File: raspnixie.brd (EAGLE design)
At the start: 87.6 x 58.5 mm, 30 parts, among them IC1 74141N, IC2 74141N, IC3 74141N, IC4 74141N, T1 IRF644B, T2 13001, U1 ZM1000, U2 ZM1000, U3 ZM1000, U4 ZM1000, U5 MAX1771CPA+, X1 RASPI_BOARD_B+#_E3P

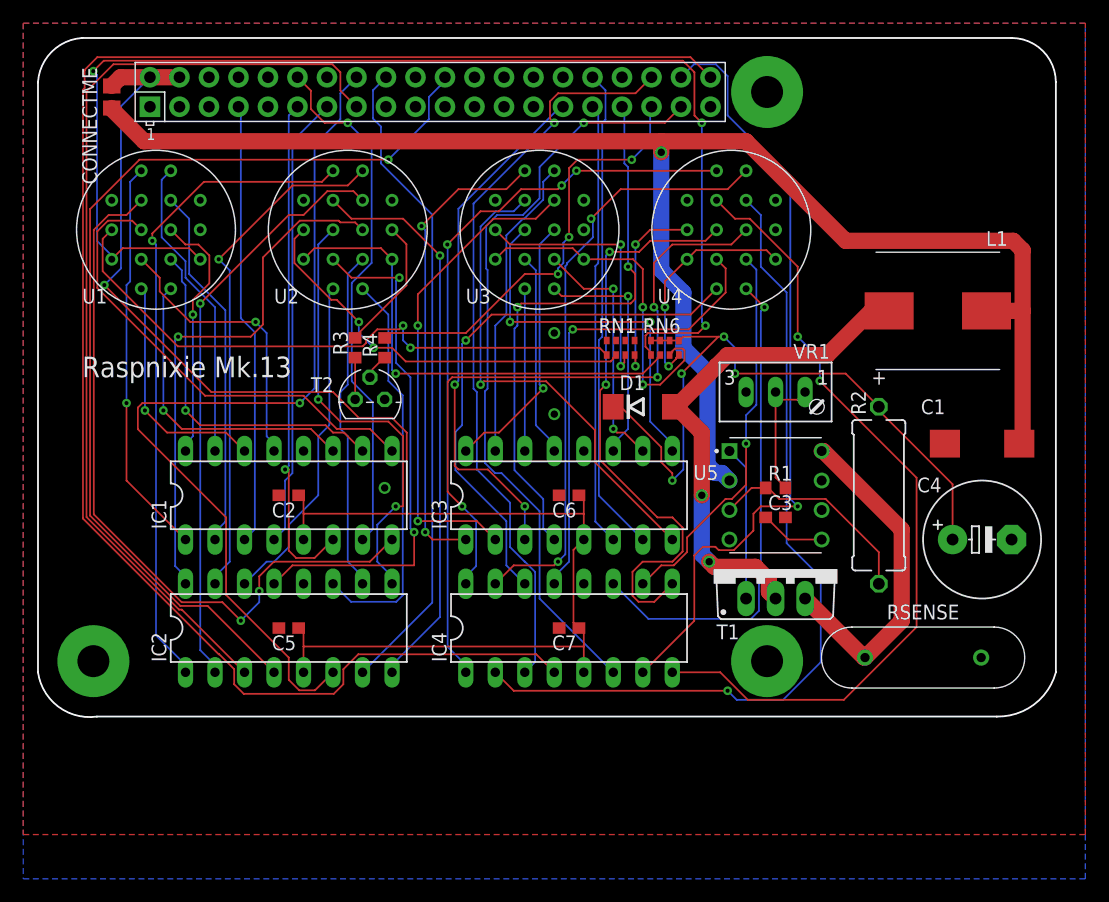
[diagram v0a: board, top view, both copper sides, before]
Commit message: mark. 14
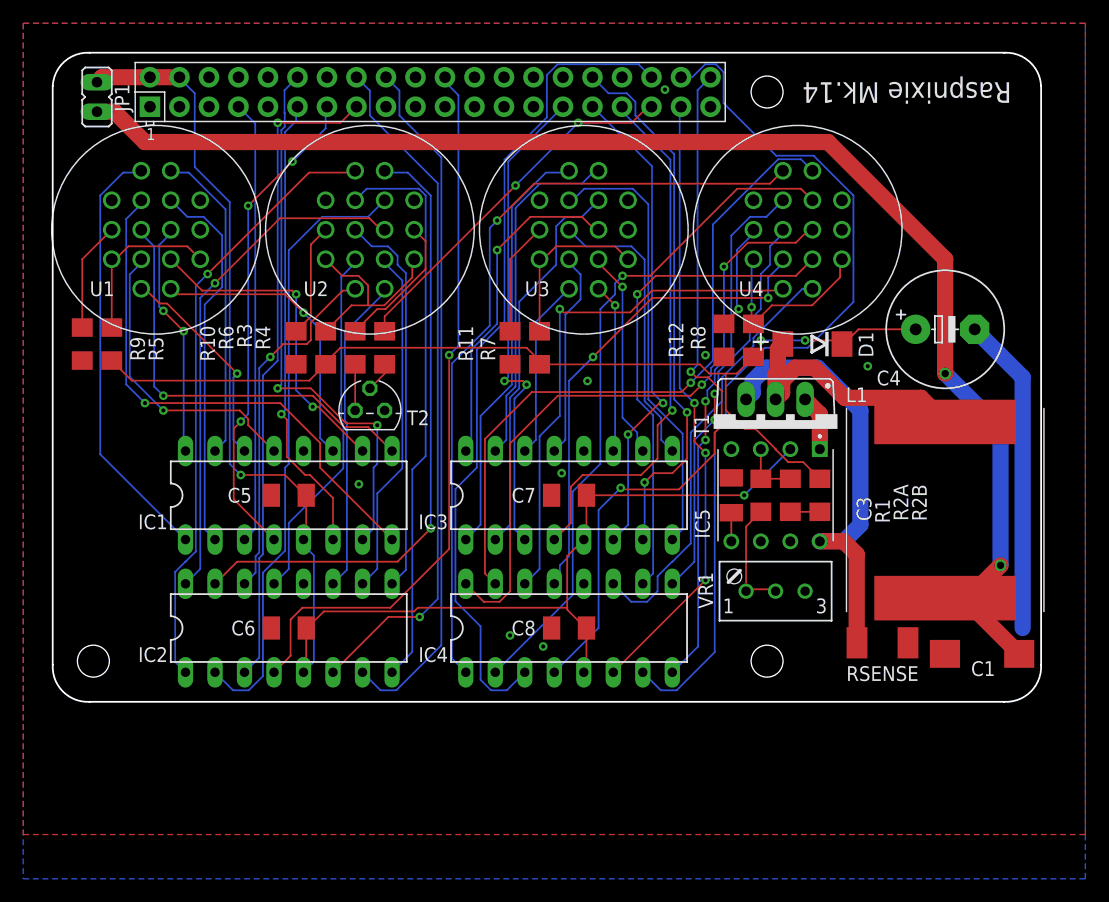
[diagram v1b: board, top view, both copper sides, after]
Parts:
- removed C2: 10n, rcl:C0603
- removed CONNECTME: 0, rcl:R0805
- removed R2: 1M5, rcl:P0613/15
- removed RN1: 10M, resistor-dil:0603-ARC
- removed RN6: 18k, resistor-dil:0603-ARV
- added C8: 10n, rcl:C1206K
- added JP1: (no value), jumper:JP1
- added R10, R11, R12, R9: 10M, rcl:R1206
- added R2A, R2B: 750k, rcl:R1206
- added R5, R6, R7, R8: 15k, rcl:R1206
- C3, C5, C6, C7: device rcl:C0603 -> rcl:C1206K
- L1: value 101 -> 221; device raspnixie:INDM106101X500N -> raspnixie:RESM175170X700N
- R1, R3, R4: device rcl:R0603 -> rcl:R1206
- RSENSE: device raspnixie:XTALRR1000W60L1750T525H1800B -> rcl:R2010
- VR1: device pot:S64W -> pot-hex:S64W-ROUND
- X1: value RASPI_BOARD_B+#_E3P -> RASPI_BOARD_B+#_E3; device raspberrypi_bastelstube_v13:RASPI_BOARD_B+_EDGES_3DRILL_PAD -> raspberrypi_bastelstube_v13:RASPI_BOARD_B+_EDGES_3DRILL
- moved C6 26.7 mm to (21.6, 7.62)
- moved C4 18.4 mm to (78.1, 33.3)
- moved C1 18.1 mm to (81.3, 5.40)
- moved L1 17.2 mm to (78.1, 17.8), turned to 90 degrees
- moved D1 15.6 mm to (66.7, 32.1), turned to 180 degrees
- moved VR1 14.6 mm to (63.5, 12.1), turned to 180 degrees
- moved T1 12.1 mm to (63.5, 24.8), turned to 180 degrees
- moved C5 11.4 mm to (21.6, 19.1)
- moved C7 11.4 mm to (45.7, 19.1)
- moved U4 5.72 mm to (65.4, 41.9)
- moved C3 4.26 mm to (59.7, 19.1), turned to 90 degrees
- moved U3 3.81 mm to (47.0, 41.9)
- moved RSENSE 3.72 mm to (72.7, 6.35)
- moved U2 1.90 mm to (28.6, 41.9)
- moved R1 1.42 mm to (62.2, 19.1), turned to 270 degrees
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- renumbered U5 to IC5
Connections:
- new net N$75: R2A.2, R2B.1
- net GND: now also C8.2, R10.2, R11.2, R12.2, R9.2; no longer C2.2, RN1.5, RN1.6, RN1.7, RN1.8
- net N$1: now also R9.1; no longer RN1.1
- net N$2: now also R10.1; no longer RN1.2
- net N$3: now also R11.1; no longer RN1.3
- net N$4: now also R12.1; no longer RN1.4
- net N$65: now also R5.1; no longer RN6.1
- net N$66: now also R6.1; no longer RN6.2
- net N$70: now also R2A.1; no longer R2.2
- net N$71: now also R7.1; no longer RN6.3
- net N$72: now also R8.1; no longer RN6.4
- net V+: now also JP1.1; no longer CONNECTME.2, IC5.2
- net VCC: now also C8.1, IC5.2, JP1.2; no longer C2.1, CONNECTME.1
- net VH: now also R2B.2, R5.2, R6.2, R7.2, R8.2; no longer R2.1, RN6.5, RN6.6, RN6.7, RN6.8
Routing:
- net N$65: track 107.4 -> 14.4 mm, vias 3 -> 0
- net N$60: track 144.3 -> 62.7 mm, vias 0 -> 2
- net N$1: track 52.6 -> 9.47 mm, vias 2 -> 0
- net VH: track 60.6 -> 89.1 mm, vias 4 -> 2
- net GND: track 0.08 -> 27.4 mm, vias 3 -> 8
- net N$64: track 82.4 -> 55.8 mm, vias 0 -> 1
- net N$2: track 35.2 -> 9.79 mm, vias 2 -> 0
- net N$66: track 41.9 -> 17.3 mm, vias 1 -> 0
- net N$38: track 69.2 -> 45.4 mm
- net N$52: track 84.4 -> 62.7 mm
- net N$62: track 44.2 -> 23.3 mm, vias 2 -> 0
- net N$50: track 77.8 -> 59.4 mm
- net N$8: track 63.3 -> 46.1 mm, vias 2 -> 1
- net N$39: track 51.2 -> 34.4 mm
- net N$71: track 30.7 -> 14.7 mm, vias 2 -> 0
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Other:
- board size 87.6 x 58.5 mm -> 85.1 x 55.9 mm
- board text added: "Raspnixie Mk.14"
- board text removed: "Raspnixie Mk.13"

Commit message: steal from other libraries
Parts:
- IC1, IC2, IC3, IC4: device 74xx-eu:DIL16 -> raspnixie:DIL16
- IC5: device MAX1771CPA:DIP794W47P254L991H457Q8 -> raspnixie:DIP794W47P254L991H457Q8
- T1: device Transistor:TO220BV -> transistor-power:TO220BV
- T2: value 13001 -> A42; device Transistor:TO92 -> transistor:TO92
- VR1: device pot-hex:S64W-ROUND -> raspnixie:S64W-ROUND
- X1: device raspberrypi_bastelstube_v13:RASPI_BOARD_B+_EDGES_3DRILL -> raspnixie:RASPI_BOARD_B+_EDGES_3DRILL
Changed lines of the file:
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@@
 <drawing>
 <settings>
-<setting alwaysvectorfont="yes"/>
+<setting alwaysvectorfont="no"/>
 <setting verticaltext="up"/>
 </settings>
@@
 </autorouter>
 <elements>
-<element name="X1" library="raspberrypi_bastelstube_v13" package="RASPI_BOARD_B+_EDGES_3DRILL" value="RASPI_BOARD_B+#_E3" x="1.27" y="1.27" smashed="yes">
+<element name="X1" library="raspnixie" package="RASPI_BOARD_B+_EDGES_3DRILL" value="RASPI_BOARD_B+#_E3" x="1.27" y="1.27" smashed="yes">
 <attribute name="SPICEPREFIX" value="X" x="1.27" y="1.27" size="1.778" layer="27" display="off"/>
 </element>
-<element name="IC1" library="74xx-eu" library_urn="urn:adsk.eagle:library:85" package="DIL16" package3d_urn="urn:adsk.eagle:package:922/2" value="74141N" x="21.59" y="19.05" smashed="yes">
+<element name="IC1" library="raspnixie" package="DIL16" package3d_urn="urn:adsk.eagle:package:922/2" value="74141N" x="21.59" y="19.05" smashed="yes">
 <attribute name="NAME" x="11.176" y="17.399" size="1.27" layer="25" ratio="10" rot="R180"/>
 <attribute name="POPULARITY" value="0" x="21.59" y="34.29" size="1.778" layer="27" display="off"/>
@@
 <attribute name="NAME" x="4.445" y="36.195" size="1.27" layer="21"/>
 </element>
-<element name="IC2" library="74xx-eu" library_urn="urn:adsk.eagle:library:85" package="DIL16" package3d_urn="urn:adsk.eagle:package:922/2" value="74141N" x="21.59" y="7.62" smashed="yes">
+<element name="IC2" library="raspnixie" package="DIL16" package3d_urn="urn:adsk.eagle:package:922/2" value="74141N" x="21.59" y="7.62" smashed="yes">
 <attribute name="NAME" x="11.176" y="5.969" size="1.27" layer="25" ratio="10" rot="R180"/>
 <attribute name="POPULARITY" value="0" x="21.59" y="21.59" size="1.778" layer="27" display="off"/>
@@
 <attribute name="NAME" x="22.86" y="36.195" size="1.27" layer="21"/>
 </element>
-<element name="IC3" library="74xx-eu" library_urn="urn:adsk.eagle:library:85" package="DIL16" package3d_urn="urn:adsk.eagle:package:922/2" value="74141N" x="45.72" y="19.05" smashed="yes">
+<element name="IC3" library="raspnixie" package="DIL16" package3d_urn="urn:adsk.eagle:package:922/2" value="74141N" x="45.72" y="19.05" smashed="yes">
 <attribute name="NAME" x="35.306" y="17.399" size="1.27" layer="25" ratio="10" rot="R180"/>
 <attribute name="POPULARITY" value="0" x="45.72" y="33.02" size="1.778" layer="27" display="off"/>
@@
 <attribute name="NAME" x="41.91" y="36.195" size="1.27" layer="21"/>
 </element>
-<element name="IC4" library="74xx-eu" library_urn="urn:adsk.eagle:library:85" package="DIL16" package3d_urn="urn:adsk.eagle:package:922/2" value="74141N" x="45.72" y="7.62" smashed="yes">
+<element name="IC4" library="raspnixie" package="DIL16" package3d_urn="urn:adsk.eagle:package:922/2" value="74141N" x="45.72" y="7.62" smashed="yes">
 <attribute name="NAME" x="35.306" y="5.969" size="1.27" layer="25" ratio="10" rot="R180"/>
 <attribute name="POPULARITY" value="0" x="45.72" y="21.59" size="1.778" layer="27" display="off"/>
@@
 <attribute name="NAME" x="60.325" y="36.195" size="1.27" layer="21"/>
 </element>
-<element name="IC5" library="MAX1771CPA" package="DIP794W47P254L991H457Q8" value="MAX1771CPA+" x="63.5" y="19.05" smashed="yes" rot="R270">
+<element name="IC5" library="raspnixie" package="DIP794W47P254L991H457Q8" value="MAX1771CPA+" x="63.5" y="19.05" smashed="yes" rot="R270">
 <attribute name="AVAILABILITY" value="Unavailable" x="63.5" y="19.05" size="1.778" layer="27" rot="R270" display="off"/>
 <attribute name="DESCRIPTION" value=" Boost, Buck-Boost Regulator Positive Output Step-Up, Step-Up/Step-Down DC-DC Controller IC 8-PDIP " x="63.5" y="19.05" size="1.778" layer="27" rot="R270" display="off"/>
@@
 <attribute name="VALUE" x="83.82" y="9.2075" size="1.27" layer="27" rot="R180"/>
 </element>
-<element name="T1" library="Transistor" library_urn="urn:adsk.eagle:library:16378713" package="TO220BV" package3d_urn="urn:adsk.eagle:package:29484/3" value="IRF644B" x="63.5" y="24.765" smashed="yes" rot="R180">
-<attribute name="CATEGORY" value="Transistor" x="63.5" y="24.765" size="1.778" layer="27" rot="R180" display="off"/>
-<attribute name="DESCRIPTION" value="" x="63.5" y="24.765" size="1.778" layer="27" rot="R180" display="off"/>
-<attribute name="DRAIN_CURRENT" value="" x="63.5" y="24.765" size="1.778" layer="27" rot="R180" display="off"/>
-<attribute name="MANUFACTURER" value="" x="63.5" y="24.765" size="1.778" layer="27" rot="R180" display="off"/>
-<attribute name="MPN" value="" x="63.5" y="24.765" size="1.778" layer="27" rot="R180" display="off"/>
+<element name="T1" library="transistor-power" library_urn="urn:adsk.eagle:library:400" package="TO220BV" package3d_urn="urn:adsk.eagle:package:29484/3" value="IRF644B" x="63.5" y="24.765" smashed="yes" rot="R180">
 <attribute name="NAME" x="56.5023" y="26.035" size="1.27" layer="25" ratio="10" rot="R270"/>
-<attribute name="OPERATING_TEMP" value="" x="63.5" y="24.765" size="1.778" layer="27" rot="R180" display="off"/>
-<attribute name="PART_STATUS" value="" x="63.5" y="24.765" size="1.778" layer="27" rot="R180" display="off"/>
-<attribute name="ROHS_COMPLIANT" value="" x="63.5" y="24.765" size="1.778" layer="27" rot="R180" display="off"/>
-<attribute name="SERIES" value="" x="63.5" y="24.765" size="1.778" layer="27" rot="R180" display="off"/>
-<attribute name="SUB-CATEGORY" value="MOSFET" x="63.5" y="24.765" size="1.778" layer="27" rot="R180" display="off"/>
-<attribute name="THERMALLOSS" value="" x="63.5" y="24.765" size="1.778" layer="27" rot="R180" display="off"/>
-<attribute name="TYPE" value="N-Channel" x="63.5" y="24.765" size="1.778" layer="27" rot="R180" display="off"/>
+<attribute name="POPULARITY" value="7" x="63.5" y="24.765" size="1.778" layer="27" rot="R180" display="off"/>
 <attribute name="VALUE" x="68.58" y="32.385" size="1.27" layer="27" ratio="10" rot="R180"/>
 </element>
@@
 <attribute name="VALUE" x="60.325" y="19.685" size="1.27" layer="27" rot="R270"/>
 </element>
-<element name="VR1" library="pot-hex" package="S64W-ROUND" value="5k" x="63.5" y="12.065" smashed="yes" rot="R180">
+<element name="VR1" library="raspnixie" package="S64W-ROUND" value="5k" x="63.5" y="12.065" smashed="yes" rot="R180">
 <attribute name="NAME" x="56.8452" y="12.446" size="1.27" layer="25" ratio="10" rot="R270"/>
 <attribute name="VALUE" x="68.3006" y="14.986" size="1.27" layer="27" ratio="10" rot="R180"/>
@@
 <attribute name="VALUE" x="69.315" y="34.7735" size="1.27" layer="27" ratio="10" rot="R180"/>
 </element>
-<element name="T2" library="Transistor" library_urn="urn:adsk.eagle:library:16378713" package="TO92" package3d_urn="urn:adsk.eagle:package:16378726/1" value="13001" x="28.575" y="26.3525" smashed="yes">
-<attribute name="CATEGORY" value="Transistor" x="28.575" y="26.3525" size="1.778" layer="27" display="off"/>
-<attribute name="DESCRIPTION" value="" x="28.575" y="26.3525" size="1.778" layer="27" display="off"/>
-<attribute name="IC_MAX" value="" x="28.575" y="26.3525" size="1.778" layer="27" display="off"/>
-<attribute name="MANUFACTURER" value="" x="28.575" y="26.3525" size="1.778" layer="27" display="off"/>
-<attribute name="MPN" value="" x="28.575" y="26.3525" size="1.778" layer="27" display="off"/>
+<element name="T2" library="transistor" library_urn="urn:adsk.eagle:library:402" package="TO92" package3d_urn="urn:adsk.eagle:package:28523/2" value="A42" x="28.575" y="26.3525" smashed="yes">
 <attribute name="NAME" x="31.75" y="25.0825" size="1.27" layer="25" ratio="10"/>
-<attribute name="OPERATING_TEMP" value="" x="28.575" y="26.3525" size="1.778" layer="27" display="off"/>
-<attribute name="PART_STATUS" value="" x="28.575" y="26.3525" size="1.778" layer="27" display="off"/>
-<attribute name="ROHS_COMPLIANT" value="" x="28.575" y="26.3525" size="1.778" layer="27" display="off"/>
-<attribute name="SERIES" value="" x="28.575" y="26.3525" size="1.778" layer="27" display="off"/>
-<attribute name="SUB-CATEGORY" value="BJT" x="28.575" y="26.3525" size="1.778" layer="27" display="off"/>
-<attribute name="THERMALLOSS" value="" x="28.575" y="26.3525" size="1.778" layer="27" display="off"/>
-<attribute name="TYPE" value="NPN" x="28.575" y="26.3525" size="1.778" layer="27" display="off"/>
+<attribute name="POPULARITY" value="0" x="28.575" y="26.3525" size="1.778" layer="27" display="off"/>
 <attribute name="VALUE" x="31.75" y="25.0825" size="1.27" layer="27" ratio="10"/>
-<attribute name="VCEO_MAX" value="" x="28.575" y="26.3525" size="1.778" layer="27" display="off"/>
 </element>
 <element name="R4" library="rcl" library_urn="urn:adsk.eagle:library:334" package="R1206" package3d_urn="urn:adsk.eagle:package:23540/2" value="10k" x="29.845" y="31.75" smashed="yes" rot="R270">
